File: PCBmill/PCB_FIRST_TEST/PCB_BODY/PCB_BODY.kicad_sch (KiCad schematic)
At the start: 5 parts, among them U1 PC817

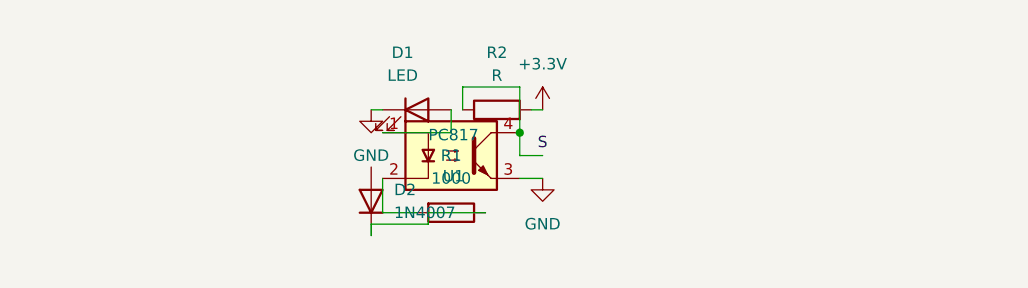
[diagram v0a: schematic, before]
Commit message: added the thhings to the stuff
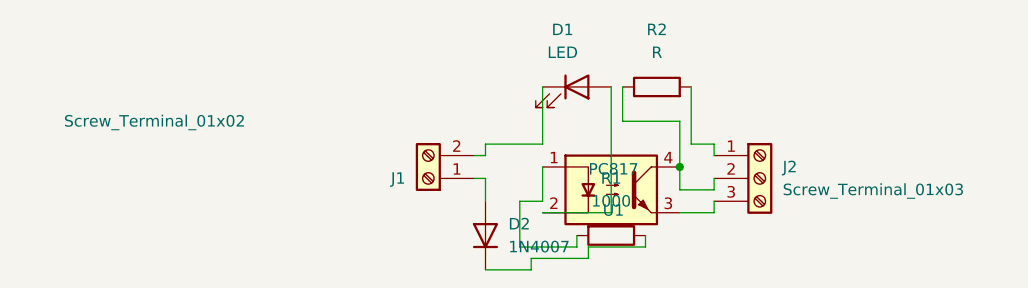
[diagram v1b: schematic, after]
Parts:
- added J1: Screw_Terminal_01x02, TerminalBlock:TerminalBlock_MaiXu_MX126-5.0-02P_1x02_P5.00mm, symbol Connector:Screw_Terminal_01x02
- added J2: Screw_Terminal_01x03, TerminalBlock:TerminalBlock_MaiXu_MX126-5.0-03P_1x03_P5.00mm, symbol Connector:Screw_Terminal_01x03
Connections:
- net at R2.1, U1.4: now also J2.2 (Pin_2)
- net at U1.1: now also R1.2; no longer D1.2 (A)
- net at U1.2: now also D1.2 (A); no longer R1.2
- net at D2.2 (A): now also J1.1 (Pin_1)
- net +3.3V: no longer names the net of R2.2
- net +3.3V: now also J2.1 (Pin_1)
- net GND: no longer names the net of D1.1 (K)
- net GND: now also J1.2 (Pin_2); no longer U1.3
- new net: J2.3 (Pin_3), U1.3
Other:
- note removed: "S"
- moved on the sheet: D1, D2, R1, R2, U1
